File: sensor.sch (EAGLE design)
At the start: 19 parts, among them IC1 MCP3008, IC3 ESP-WROOM-02

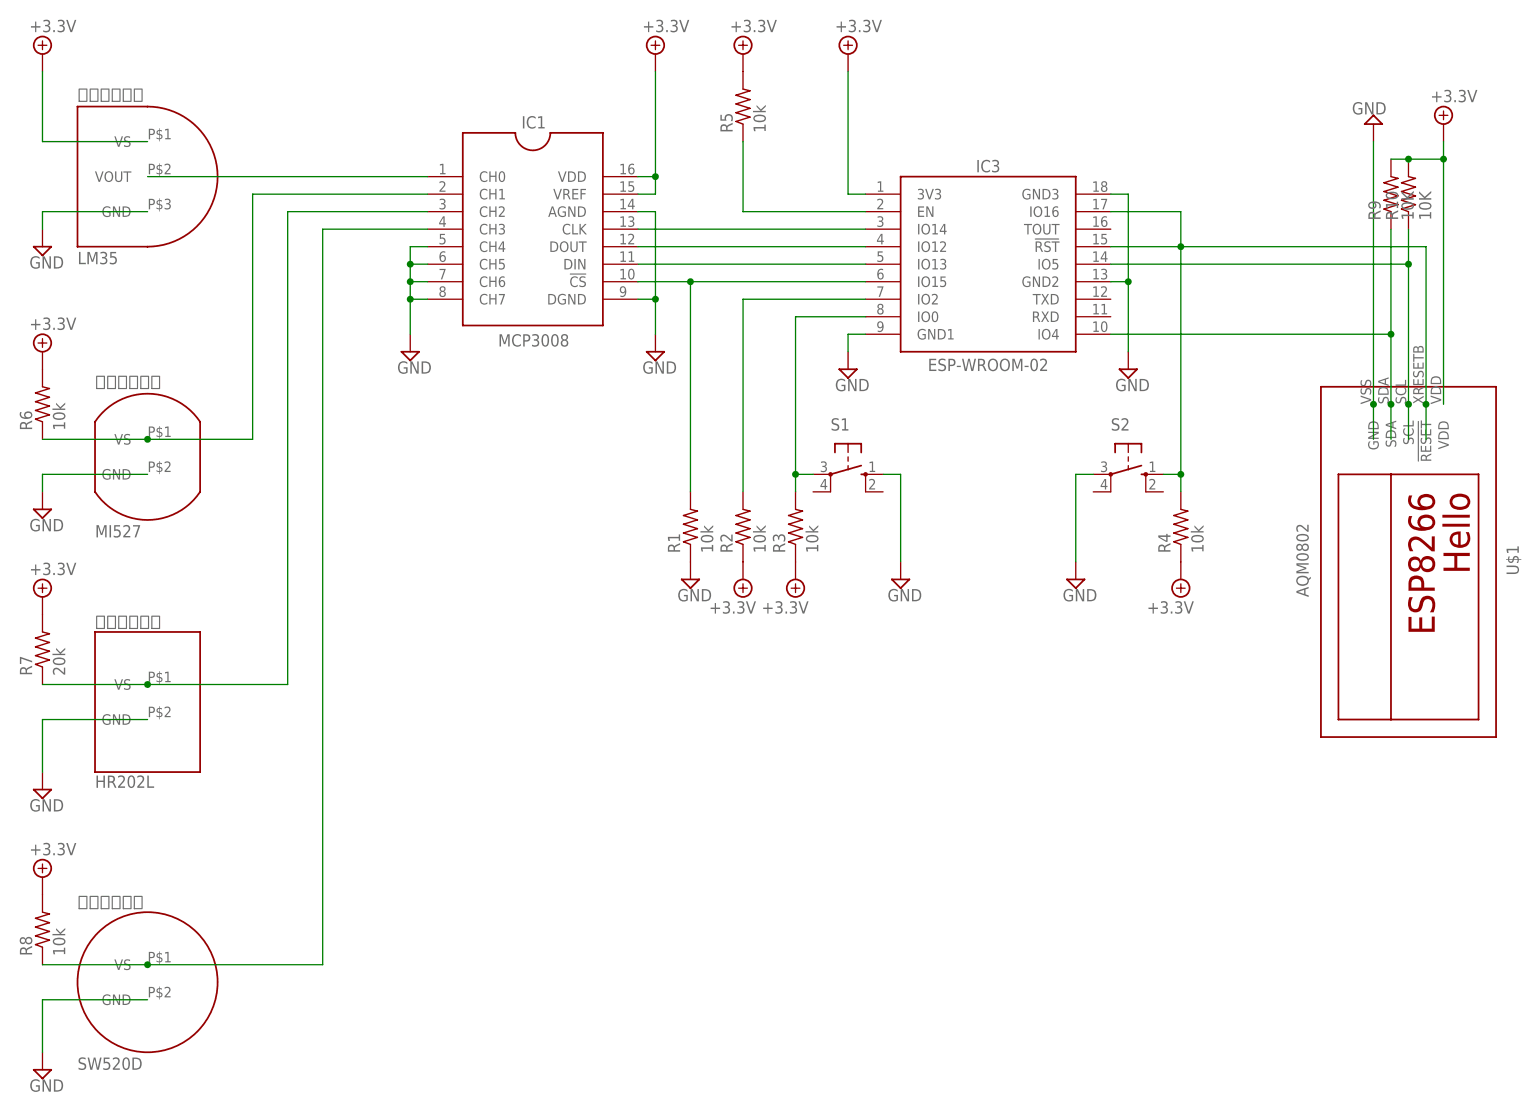
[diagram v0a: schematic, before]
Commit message: commit.
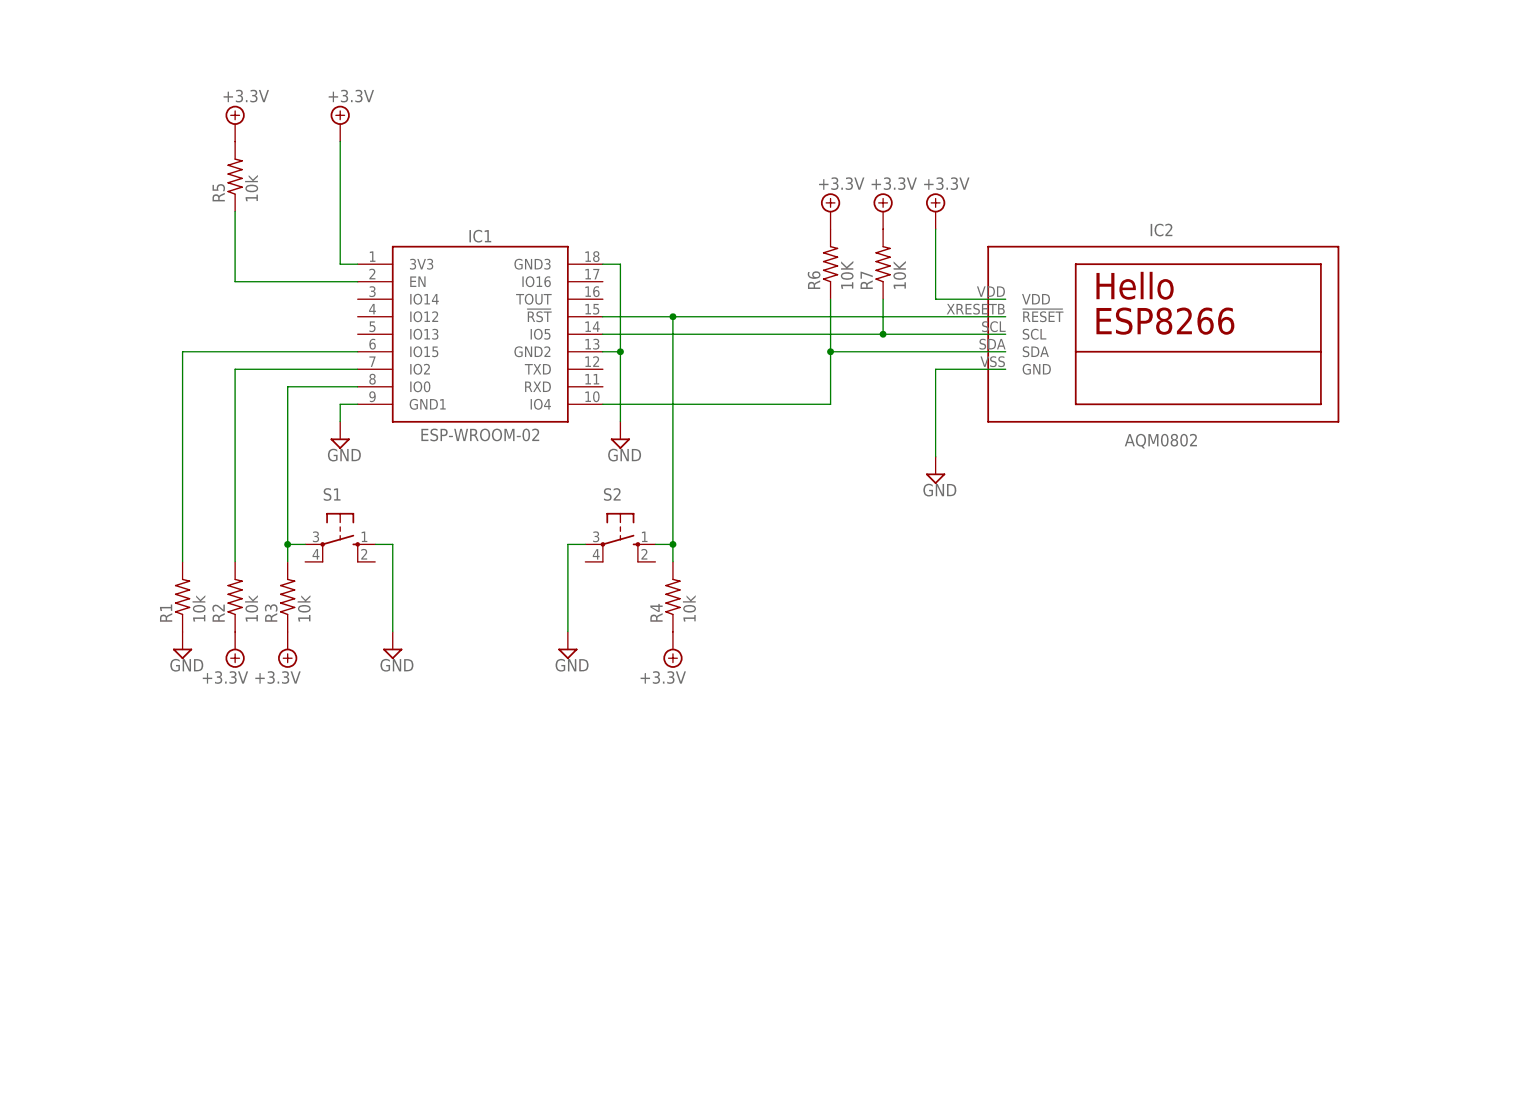
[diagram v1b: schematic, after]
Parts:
- removed IC3: ESP-WROOM-02, sensor:ESP-WROOM-02
- removed R10, R9: 10K, sensor:R
- removed R8: 10k, MyLibraries:R
- removed U$1: AQM0802, sensor:AQM0802
- removed 振動センサー: SW520D, MyLibraries:SW520D
- removed 温度センサー: LM35, MyLibraries:LM35
- removed 湿度センサー: HR202L, MyLibraries:HR202L
- removed 照度センサー: MI527, MyLibraries:MI527
- added IC2: AQM0802, sensor:AQM0802
- IC1: value MCP3008 -> ESP-WROOM-02; device sensor:MCP3008 -> sensor:ESP-WROOM-02
- R6: value 10k -> 10K; device MyLibraries:R -> sensor:R
- R7: value 20k -> 10K; device MyLibraries:R -> sensor:R
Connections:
- removed net AGND: IC1.AGND, IC1.DGND
- removed net N$11: IC1.CH0, 温度センサー.VOUT
- removed net N$12: IC1.CH2, R7.1, 湿度センサー.VS
- removed net N$13: IC1.CH3, R8.1, 振動センサー.VS
- removed net N$2: IC1.DIN, IC3.IO13
- removed net N$3: IC1.DOUT, IC3.IO12
- removed net N$6: IC1.CH1, R6.1, 照度センサー.VS
- removed net N$8: IC1.CLK, IC3.IO14
- net +3.3V: now also IC1.3V3, IC2.VDD; no longer IC1.VDD, IC1.VREF, IC3.3V3, R10.2, R8.2, R9.2, U$1.VDD, 温度センサー.VS
- net GND: now also IC2.GND; no longer IC1.CH4, IC1.CH5, IC1.CH6, IC1.CH7, U$1.GND, 振動センサー.GND, 温度センサー.GND, 湿度センサー.GND, 照度センサー.GND
- net GND1: now also IC1.GND1; no longer IC3.GND1
- net GND3: now also IC1.GND2, IC1.GND3; no longer IC3.GND2, IC3.GND3
- net N$1: now also IC1.IO15; no longer IC1.!CS!, IC3.IO15
- net N$10: now also IC1.IO0; no longer IC3.IO0
- net N$14: now also IC1.IO5, IC2.SCL, R7.1; no longer IC3.IO5, R10.1, U$1.SCL
- net N$15: now also IC1.EN; no longer IC3.EN
- net N$16: now also IC1.IO4, IC2.SDA, R6.1; no longer IC3.IO4, R9.1, U$1.SDA
- net N$5: now also IC1.IO2; no longer IC3.IO2
- net N$9: now also IC1.!RST!, IC2.!RESET!; no longer IC3.!RST!, IC3.IO16, U$1.!RESET!
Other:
- moved on the sheet: R1, R2, R3, R4, R5, R6, R7, S1, S2
